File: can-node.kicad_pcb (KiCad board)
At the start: 2 copper layers, 68.6 x 66.8 mm, 43 parts, among them J1 Conn_01x02_Pin, J10 MCP2551, J11 Conn_01x02_Socket, J13 SDA, J14 SCL, J15 MD13 SIGNAL, J17 MD13S PWR, J2 Conn_01x02_Pin, J3 CAN, J4 CAN, J5 MPU9250, J6 ENCODER, J8 CRX, J9 CTX, SW1 ADDRESS, U1 ESP32-DEVKIT-V1

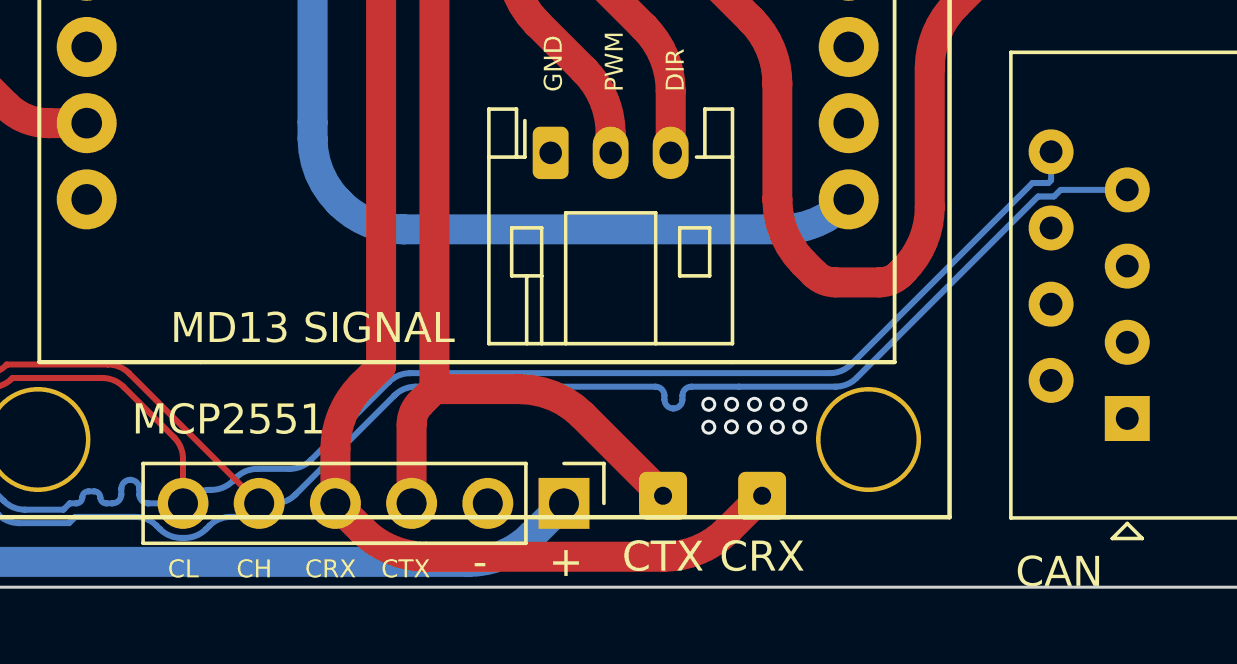
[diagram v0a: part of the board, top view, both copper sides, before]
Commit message: .
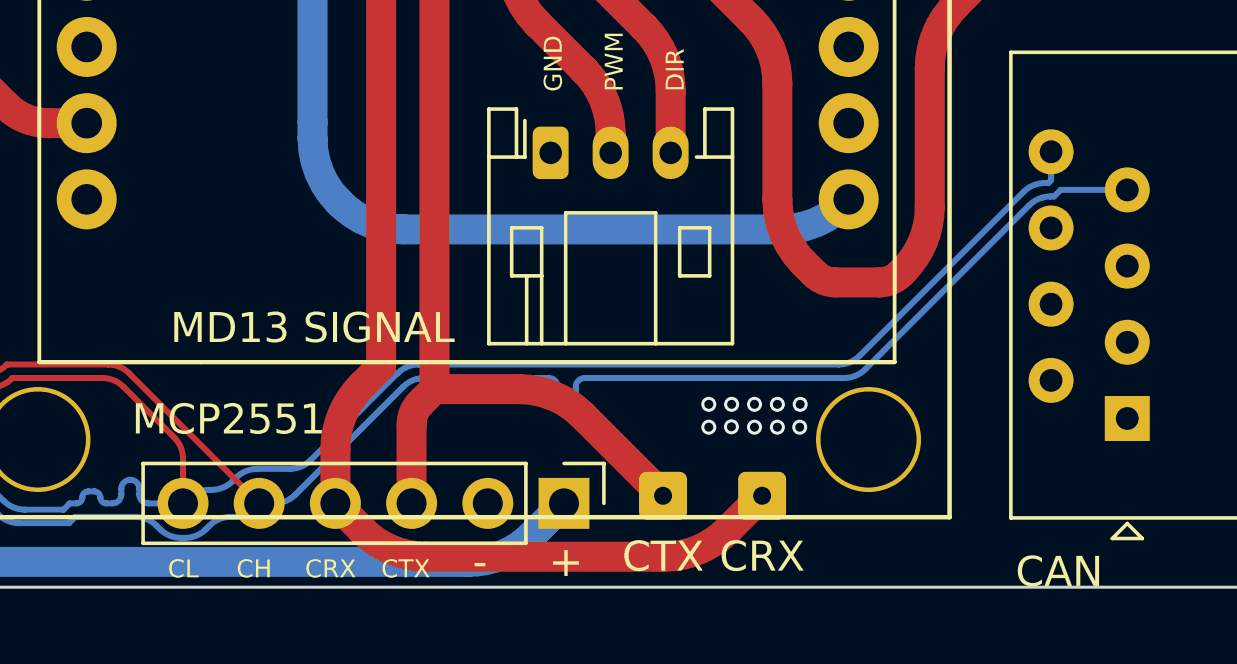
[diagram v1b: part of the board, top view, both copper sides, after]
